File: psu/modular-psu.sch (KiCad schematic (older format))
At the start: 14 parts, among them J1 CONN_02X05, U1 TSR 2-2450, U2 3V3-REG

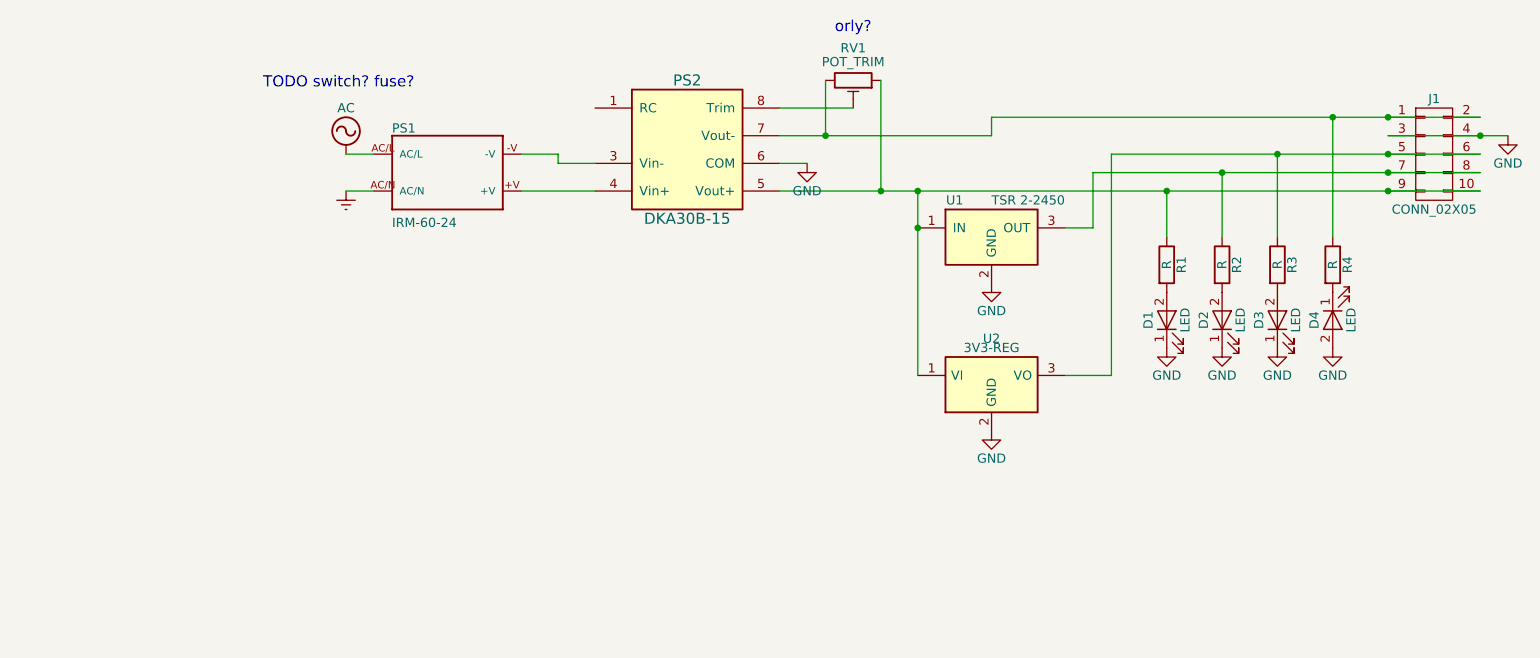
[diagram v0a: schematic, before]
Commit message: psu board
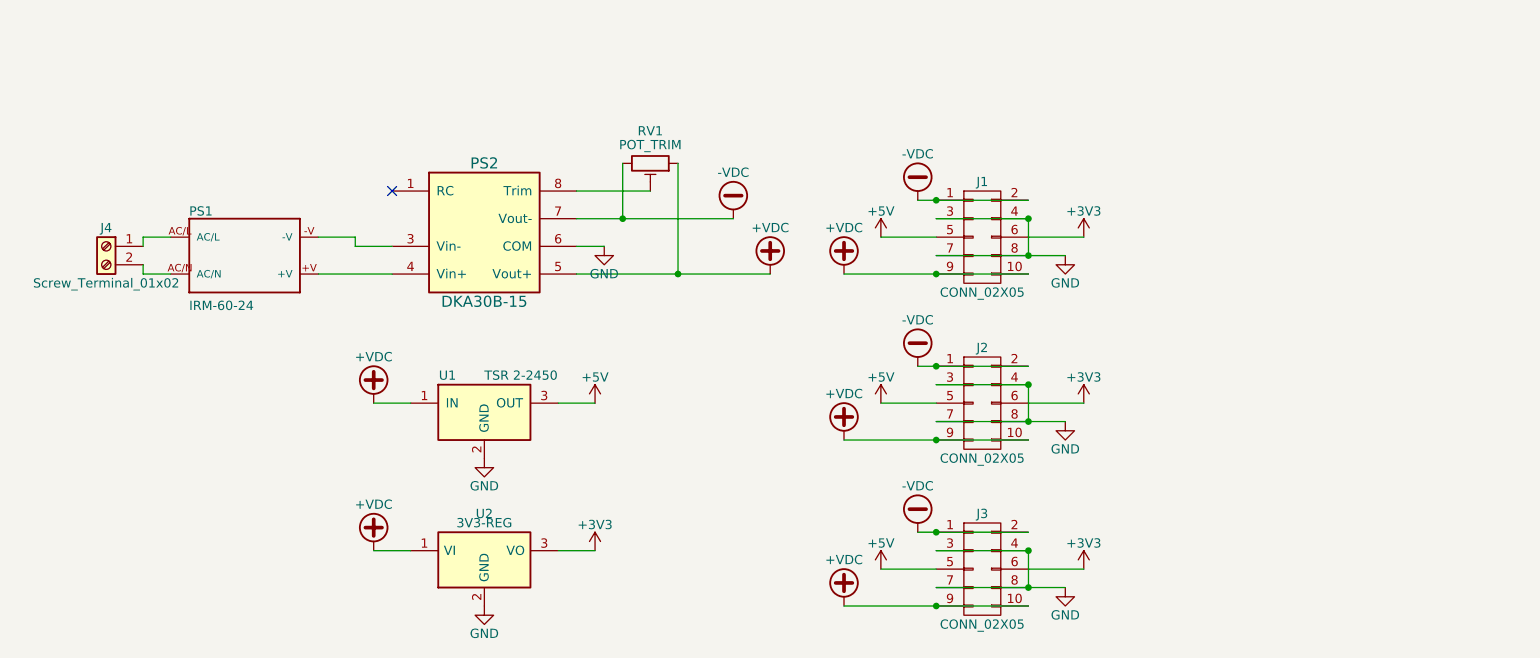
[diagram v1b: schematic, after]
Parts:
- removed D1, D2, D3, D4: LED, symbol LED
- removed R1, R2, R3, R4: R, symbol R
- added J2, J3: CONN_02X05, Pin_Headers:Pin_Header_Straight_2x05_Pitch2.54mm, symbol CONN_02X05
- added J4: Screw_Terminal_01x02, Connectors_Terminal_Blocks:TerminalBlock_Philmore_TB132_02x5mm_Straight, symbol Screw_Terminal_01x02
- J1: footprint (none) -> Pin_Headers:Pin_Header_Straight_2x05_Pitch2.54mm
- PS1: footprint CONV_IRM-60-48 -> IRM-60-24:CONV_IRM-60-48a
- PS2: footprint (none) -> dka30b-15:DKA30B-15
- RV1: footprint (none) -> Potentiometers:Potentiometer_Trimmer_Bourns_3266Y
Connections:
- net GND: now also J1.7 (P7), J1.8 (P8), J2.3 (P3), J2.4 (P4), J2.7 (P7), J2.8 (P8), J3.3 (P3), J3.4 (P4), J3.7 (P7), J3.8 (P8)
- net -VDC: now reaches J1.1 (P1), J1.2 (P2), PS2.7 (Vout-), RV1.3
- net -VDC: now also J2.1 (P1), J2.2 (P2), J3.1 (P1), J3.2 (P2)
- net +VDC: now reaches J1.10 (P10), J1.9 (P9), PS2.5 (Vout+), RV1.1, U1.1 (IN), U2.1 (VI)
- net +VDC: now also J2.10 (P10), J2.9 (P9), J3.10 (P10), J3.9 (P9)
- net +3V3: now reaches J1.6 (P6), U2.3 (VO)
- net +3V3: now also J2.6 (P6), J3.6 (P6); no longer J1.5 (P5)
- net AC: no longer names the net of PS1.AC/L
- net AC: now also J4.1 (Pin_1)
- net Earth: no longer names the net of PS1.AC/N
- net Earth: now also J4.2 (Pin_2)
- new net +5V: J1.5 (P5), J2.5 (P5), J3.5 (P5), U1.3 (OUT)
- no-connect marks 0 -> 1
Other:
- note removed: "TODO switch? fuse?"
- note removed: "orly?"
- moved on the sheet: J1, PS1, PS2, RV1, U1, U2
